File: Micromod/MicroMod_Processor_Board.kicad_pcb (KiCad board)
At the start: 4 copper layers, 32.5 x 37.5 mm, 33 parts, among them J1 MICROMOD-2222, J2 Micro_SD_Card, J3 WiFi_BT_CONN_2, J4 WiFi_BT_CONN_1, J5 TRACE, Q1 FDN340P, U1 STM32H562VGTx, Y1 ABS07AIG-32.768KHZ

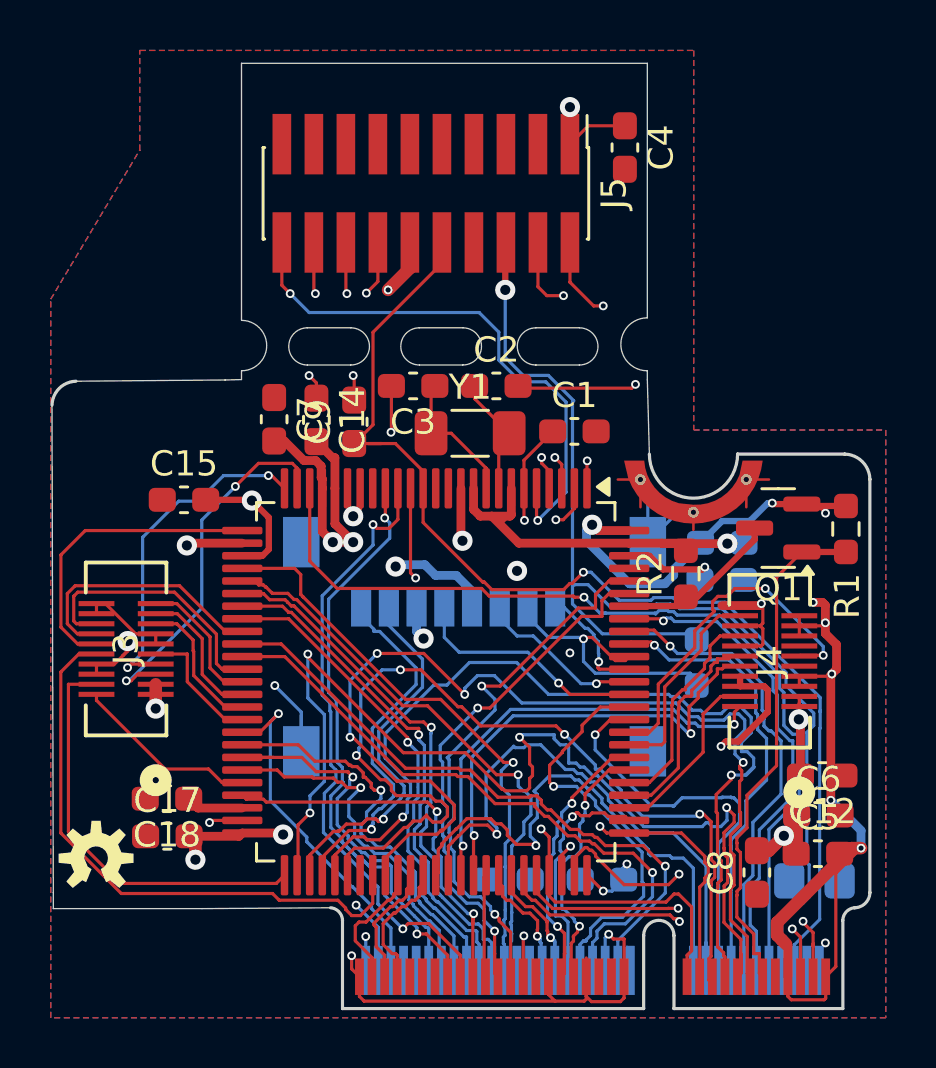
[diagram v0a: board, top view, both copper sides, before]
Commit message: almost ready for review
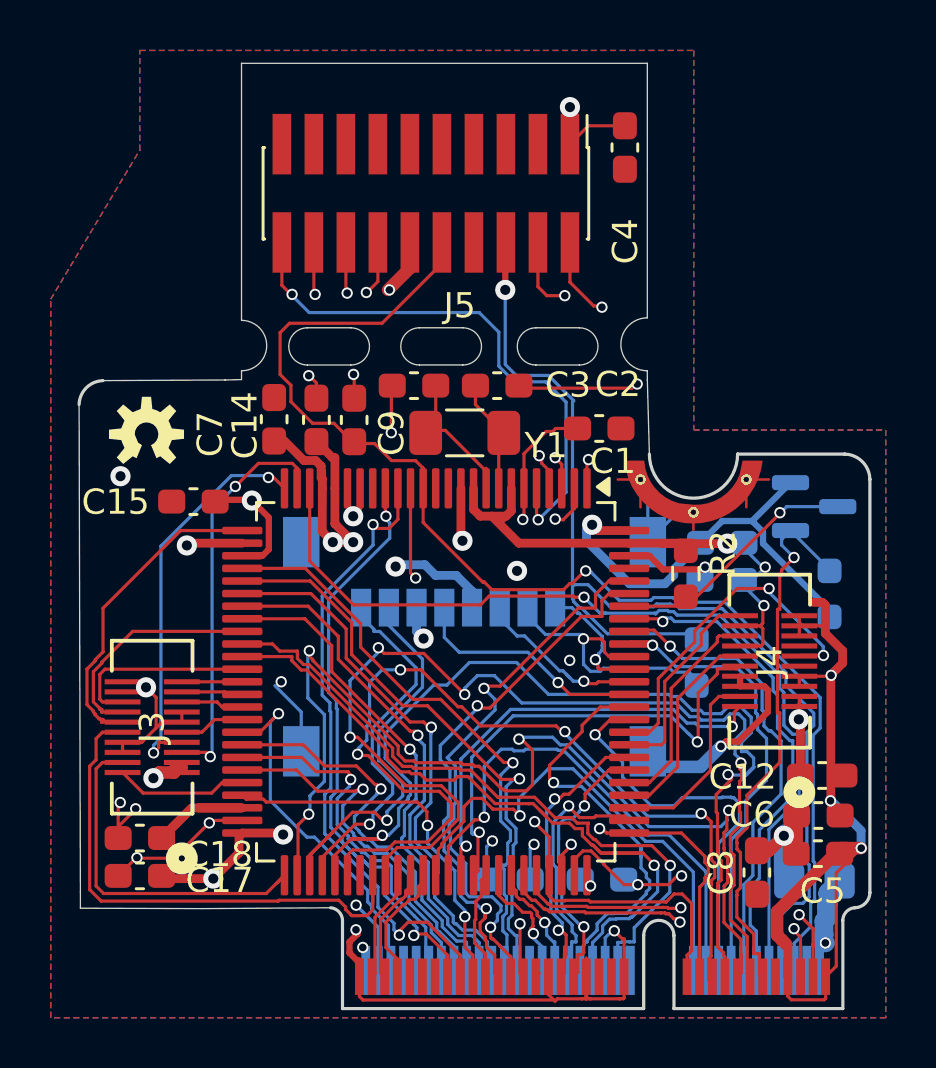
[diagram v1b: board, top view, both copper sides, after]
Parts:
- Q1, R1: moved to B.Cu
- moved LOGO3 16.9 mm to (130.8, 91.6)
- moved J3 3.27 mm to (131.0, 103.2)
- moved R1 2.66 mm to (157.9, 97.9), turned to 90 degrees
- moved C17 1.91 mm to (130.5, 109.1)
- moved C18 1.89 mm to (130.5, 107.6)
- moved Q1 1.66 mm to (157.3, 94.5), turned to 0 degrees
- moved C1 0.99 mm to (148.8, 91.3)
- moved C15 0.38 mm to (132.7, 94.2)
- moved Y1 0.22 mm to (143.4, 91.5)
- moved C9 0.07 mm to (139.0, 91.0)
- turned C16 to 180 degrees
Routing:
- net GND: track 115.7 -> 150.1 mm, vias 23 -> 28
- net +3.3V: track 147.2 -> 156.9 mm, vias 17 -> 15
- net /~{RESET}: track 45.8 -> 51.1 mm
- net Net-(C18-Pad1): track 2.27 -> 7.13 mm
- net /BOOT0: track 6.53 -> 9.92 mm, vias 0 -> 1
- net /A1: track 25.2 -> 28.6 mm
- net Net-(F1-Pad2): track 24.2 -> 27.6 mm
- net /BT_UART_RX: track 5.59 -> 2.44 mm
- net /BT_UART_RTS: track 5.61 -> 2.48 mm
- net /BT_UART_TX: track 5.44 -> 2.40 mm
- net /BT_PCM_OUT: track 10.6 -> 7.67 mm
- net /UART_RX2: track 22.8 -> 20.1 mm
- net /BT_HOST_WAKE: track 13.4 -> 16.0 mm
- net /BT_UART_CTS: track 5.16 -> 2.61 mm
- net /WL_REG_ON: track 16.5 -> 14.2 mm
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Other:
- board size 32.5 x 37.5 mm -> 31.4 x 37.5 mm
